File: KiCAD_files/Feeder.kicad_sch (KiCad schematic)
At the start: 82 parts, among them J405 Conn_01x02_Male, J406 Conn_01x02_Male, J501 Conn_01x03, Q501 60V N channel, Q502 TK13P25D,RQ, T501 PA2467NL, U407 OPA316, U501 NCP12700, U503 TL431MFDT,215

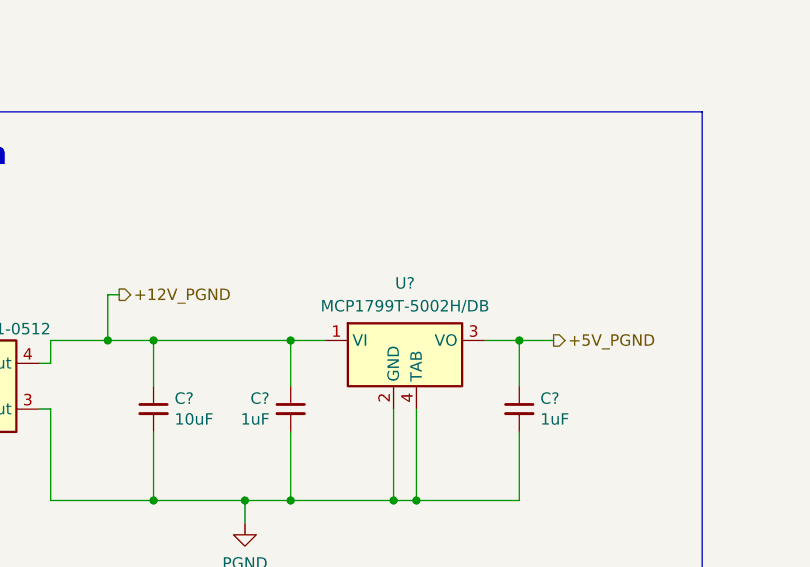
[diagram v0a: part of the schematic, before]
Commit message: ready to import netlist
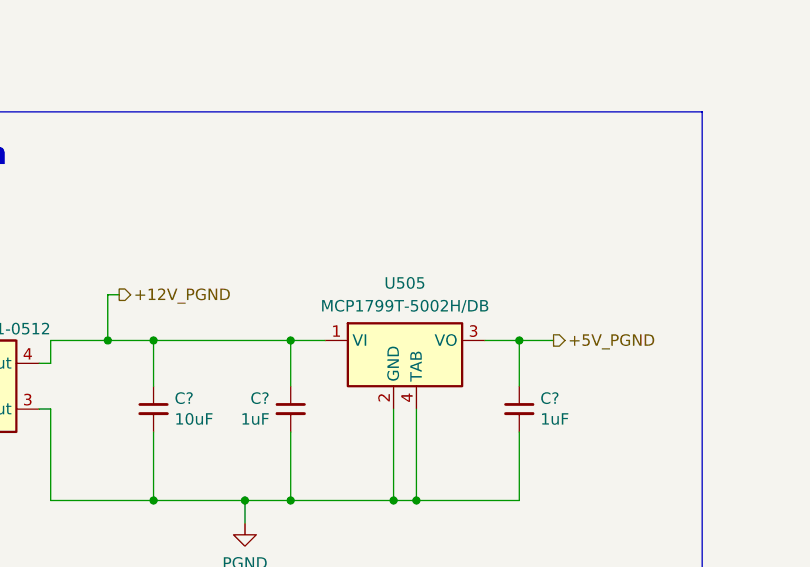
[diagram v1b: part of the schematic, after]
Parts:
- gave numbers to parts that had none: 1
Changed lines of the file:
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@@
   (symbol (lib_id "Symbols:MCP1799T-5002H/DB") (at 264.16 243.84 0) (unit 1)
     (in_bom yes) (on_board yes) (dnp no) (fields_autoplaced)
-    (property "Reference" "U?" (at 265.43 237.49 0)
+    (property "Reference" "U505" (at 265.43 237.49 0)
       (effects (font (size 1.27 1.27)))
     )
@@
       (project "ownverter"
         (path "/8d0c1d66-35ef-4a53-a28f-436a11b54f42/bce1534c-362e-45ed-a9dd-a44d6954485a"
-          (reference "U?") (unit 1)
+          (reference "U505") (unit 1)
         )
       )

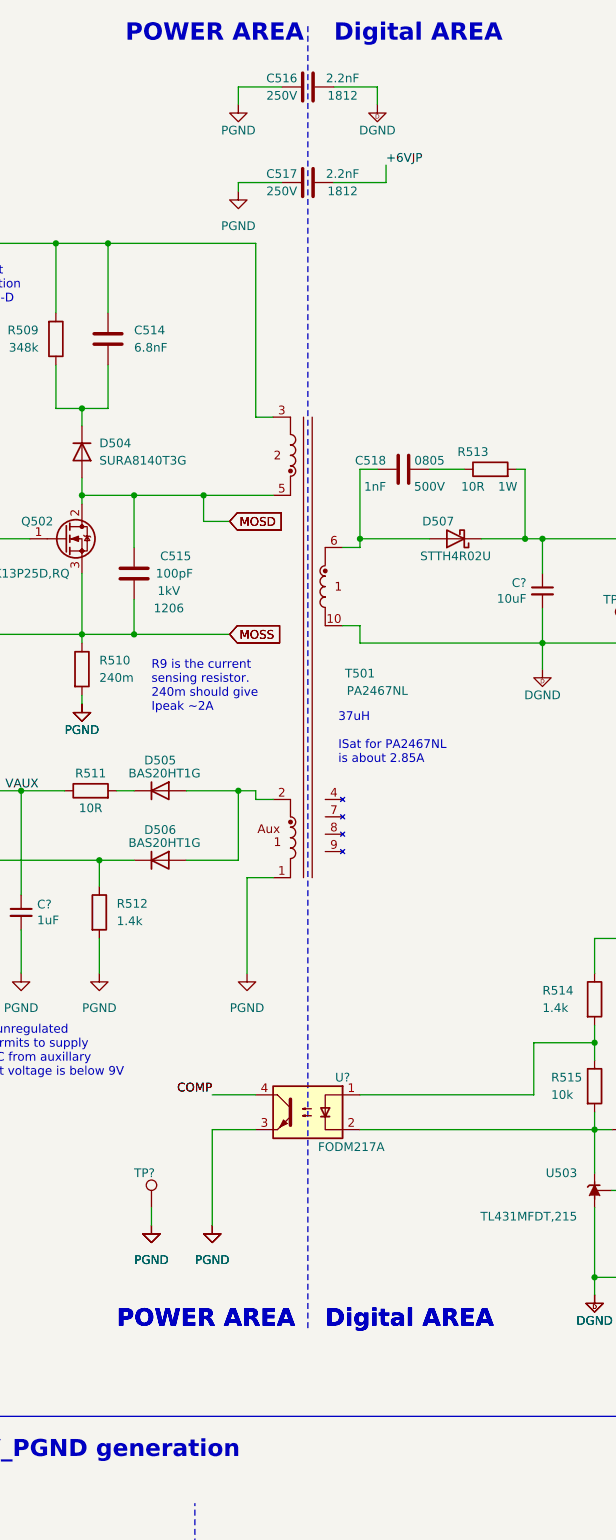
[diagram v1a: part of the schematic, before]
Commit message: WIP PCB
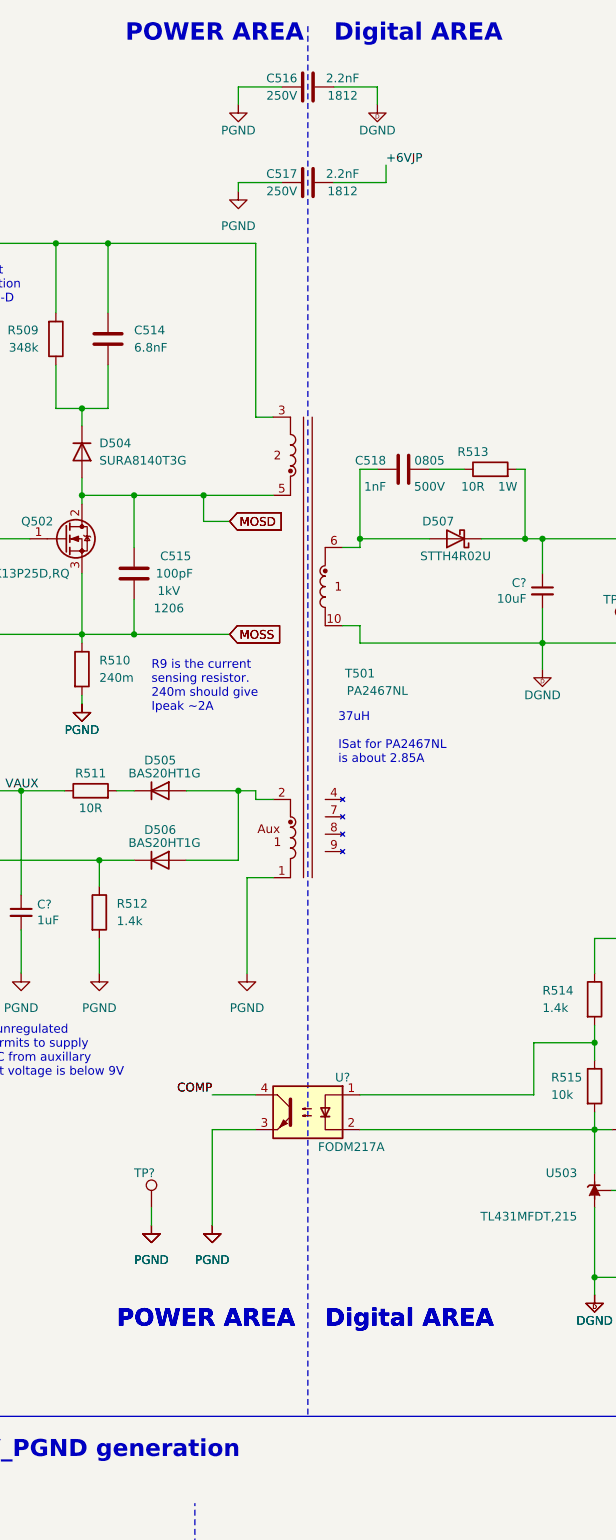
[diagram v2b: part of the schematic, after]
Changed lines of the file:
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@@
     (stroke (width 0.5) (type default))
   )
-  (polyline (pts (xy 231.14 15.24) (xy 231.14 205.74))
+  (polyline (pts (xy 231.14 15.24) (xy 231.14 218.44))
     (stroke (width 0.15) (type dash))
   )
